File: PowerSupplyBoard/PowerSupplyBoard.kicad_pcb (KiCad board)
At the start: 4 copper layers, 50 x 80 mm, 70 parts, among them J101 BATTERY, J102 POWER, J103 USB_C, J104 PWR, J105 DATA, Q101 BSH205G2A, Q102 TD6790, Q103 TD6790, Q104 TD6790, U101 TPS63021, U102 MCP73834T, U103 TC7662Bx0A, U104 TC7662Bx0A, U105 CS5173

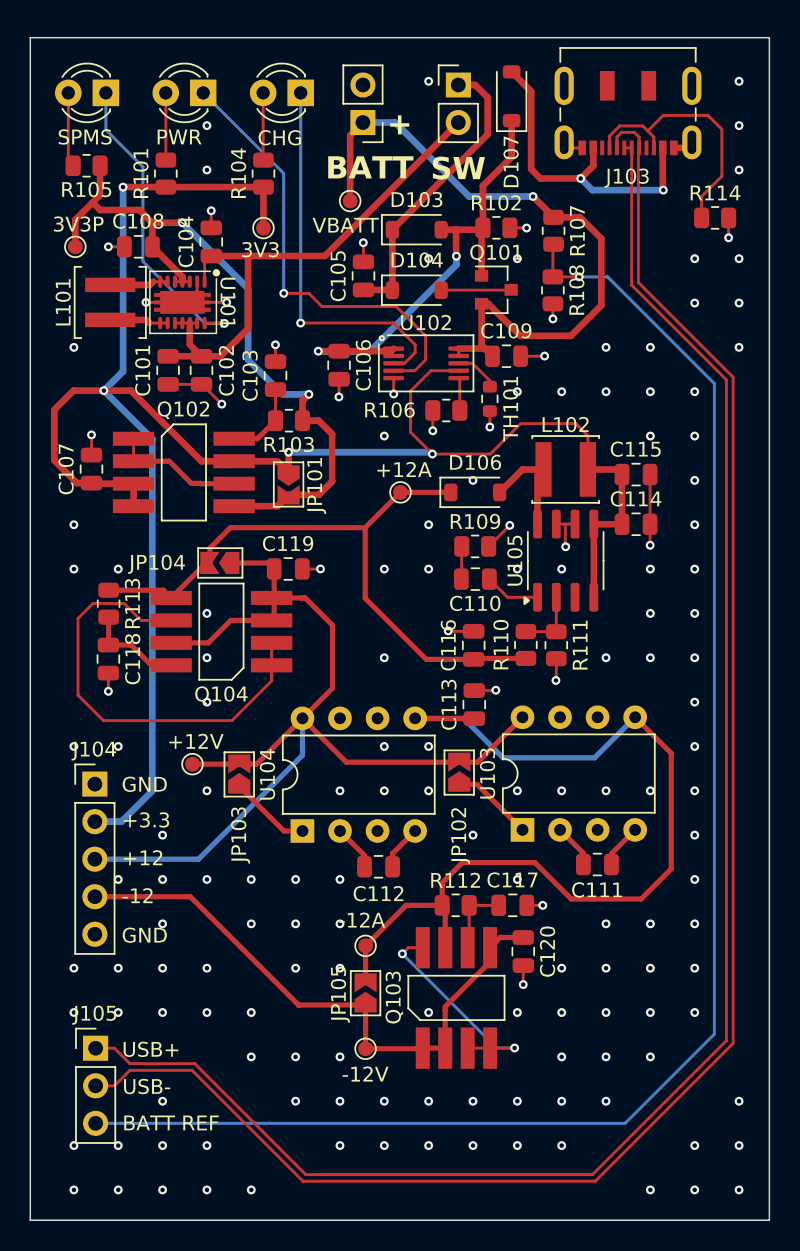
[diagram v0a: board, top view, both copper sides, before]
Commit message: Power Supply rev2
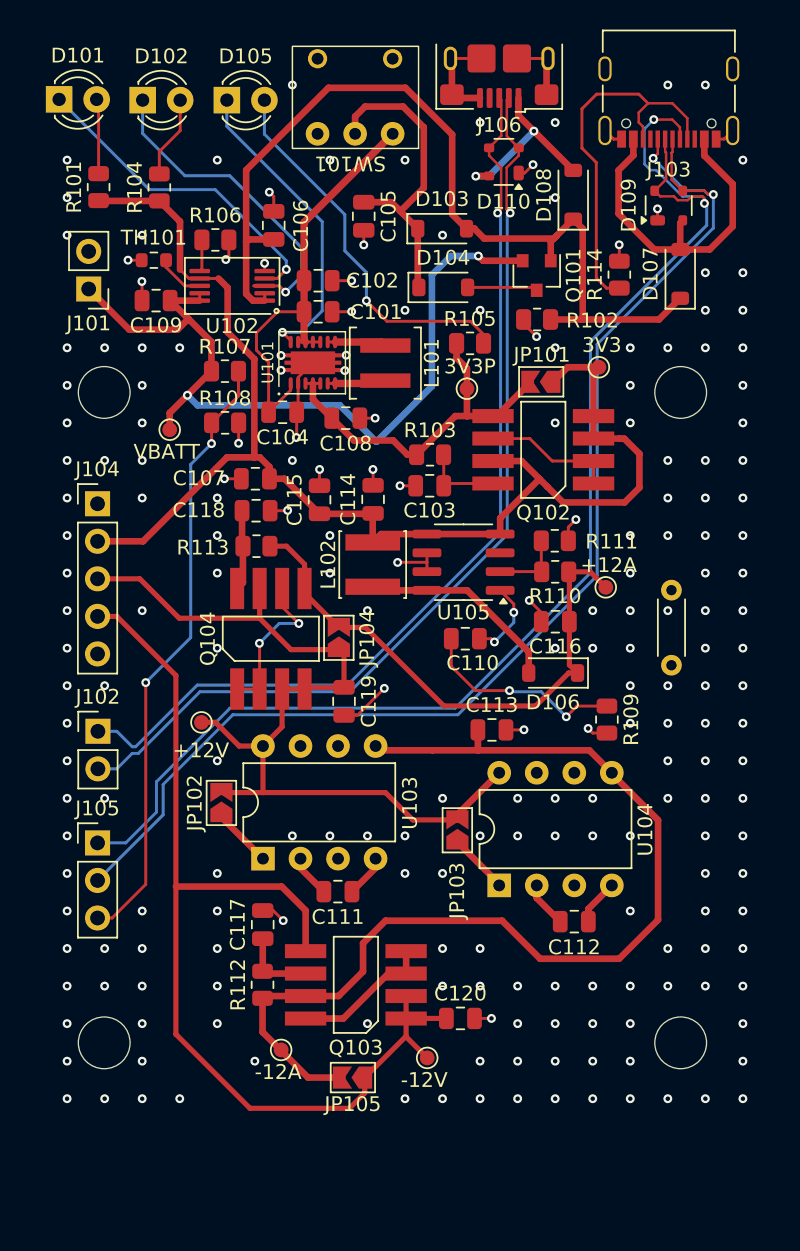
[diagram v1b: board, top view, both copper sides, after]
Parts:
- added D108: PMEG3030, Diode_SMD:D_SOD-123, F.Cu at (36.7, 10.6)
- added D109: SP0503BAHT, Package_TO_SOT_SMD:SOT-143, F.Cu at (43.2, 11.4)
- added D110: SP0503BAHT, Package_TO_SOT_SMD:SOT-143, F.Cu at (32.0, 8.40)
- added J106: USB_B_Micro, Connector_USB:USB_Micro-B_Amphenol_10118193-0001LF_Horizontal, F.Cu at (31.7, 1.41)
- added R115: LOOP, Resistor_THT:R_Axial_DIN0204_L3.6mm_D1.6mm_P5.08mm_Horizontal, F.Cu at (43.4, 42.5)
- added REF**: MountingHole_3.5mm, MountingHole:MountingHole_3.5mm, F.Cu at (44.0, 24.0)
- added REF**: MountingHole_3.5mm, MountingHole:MountingHole_3.5mm, F.Cu at (44.0, 68.0)
- added REF**: MountingHole_3.5mm, MountingHole:MountingHole_3.5mm, F.Cu at (5.00, 68.0)
- added REF**: MountingHole_3.5mm, MountingHole:MountingHole_3.5mm, F.Cu at (5.00, 24.0)
- added SW101: SW_SPDT, Button_Switch_THT:SW_NKK_B12JH_SPDT, F.Cu at (24.5, 6.50)
- J102: value POWER -> DATA2
- J103: footprint Connector_USB:USB_C_Receptacle_JAE_DX07S016JA1R1500 -> Connector_USB:USB_C_Receptacle_Palconn_UTC16-G
- J105: value DATA -> DATA1
- moved J102 50.1 mm to (4.58, 46.9)
- moved R105 28.6 mm to (29.8, 20.7), turned to 0 degrees
- moved TP102 28.2 mm to (29.5, 23.7)
- moved TH101 24.6 mm to (8.36, 15.1), turned to 180 degrees
- moved TP101 24.6 mm to (38.5, 22.3), turned to 0 degrees
- moved Q102 24.2 mm to (34.6, 27.9), turned to 180 degrees
- moved R107 24.2 mm to (13.2, 22.6), turned to 0 degrees
- moved C109 24.0 mm to (8.51, 17.8), turned to 180 degrees
- moved R108 23.9 mm to (13.2, 26.1), turned to 0 degrees
- moved J101 21.7 mm to (3.95, 17.0)
- moved C115 21.5 mm to (19.6, 31.3), turned to 90 degrees
- moved TP103 19.7 mm to (9.43, 26.5)
- moved R106 19.4 mm to (12.5, 13.7), turned to 0 degrees
- moved L101 19.1 mm to (24.0, 22.0), turned to -90 degrees
- moved J104 19.0 mm to (4.55, 31.5)
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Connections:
- J102 pad 1: VCC -> USBM_D+
- J102 pad 2: V_PWR -> USBM_D-
- J103 pad A6: USB_D+ -> USBC_D+
- J103 pad A7: USB_D- -> USBC_D-
- J103 pad B6: USB_D+ -> USBC_D+
- J103 pad B7: USB_D- -> USBC_D-
- J105 pad 1: USB_D+ -> USBC_D-
- J105 pad 2: USB_D- -> USBC_D+
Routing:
- net USB_D-: track 117.0 -> 0.00 mm
- net USB_D+: track 113.5 -> 0.00 mm
- net USBC_D-: track 0.00 -> 89.8 mm, vias 0 -> 2
- net USBC_D+: track 0.00 -> 85.1 mm, vias 0 -> 2
- net USBM_D-: track 0.00 -> 64.7 mm, vias 0 -> 1
- net USBM_D+: track 0.00 -> 64.0 mm, vias 0 -> 1
- net BATT_REF: track 104.5 -> 41.5 mm, vias 1 -> 2
- net +3.3V: track 135.9 -> 89.8 mm, vias 4 -> 0
- net -12V: track 40.3 -> 71.2 mm
- net VDD: track 33.6 -> 62.9 mm, vias 2 -> 0
- net +3.3VP: track 49.7 -> 25.6 mm, vias 2 -> 0
- net Net-(D105-A): track 5.06 -> 25.9 mm, vias 0 -> 1
- net Net-(Q104B-B2): track 29.9 -> 10.7 mm, vias 0 -> 2
- net GND: track 46.4 -> 59.6 mm, vias 162 -> 215
- net Net-(D108-A): track 0.00 -> 12.5 mm, vias 0 -> 2
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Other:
- board outline removed
- board text removed: "+"
- board text removed: "+12"
- board text removed: "+3.3"
- board text removed: "-12"
- board text removed: "BATT"
- board text removed: "BATT REF"
- board text removed: "CHG"
- board text removed: "GND"
- board text removed: "PWR"
- board text removed: "SPMS"
- board text removed: "SW"
- board text removed: "USB+"
- board text removed: "USB-"

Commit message: Power supply rev2 gerbers
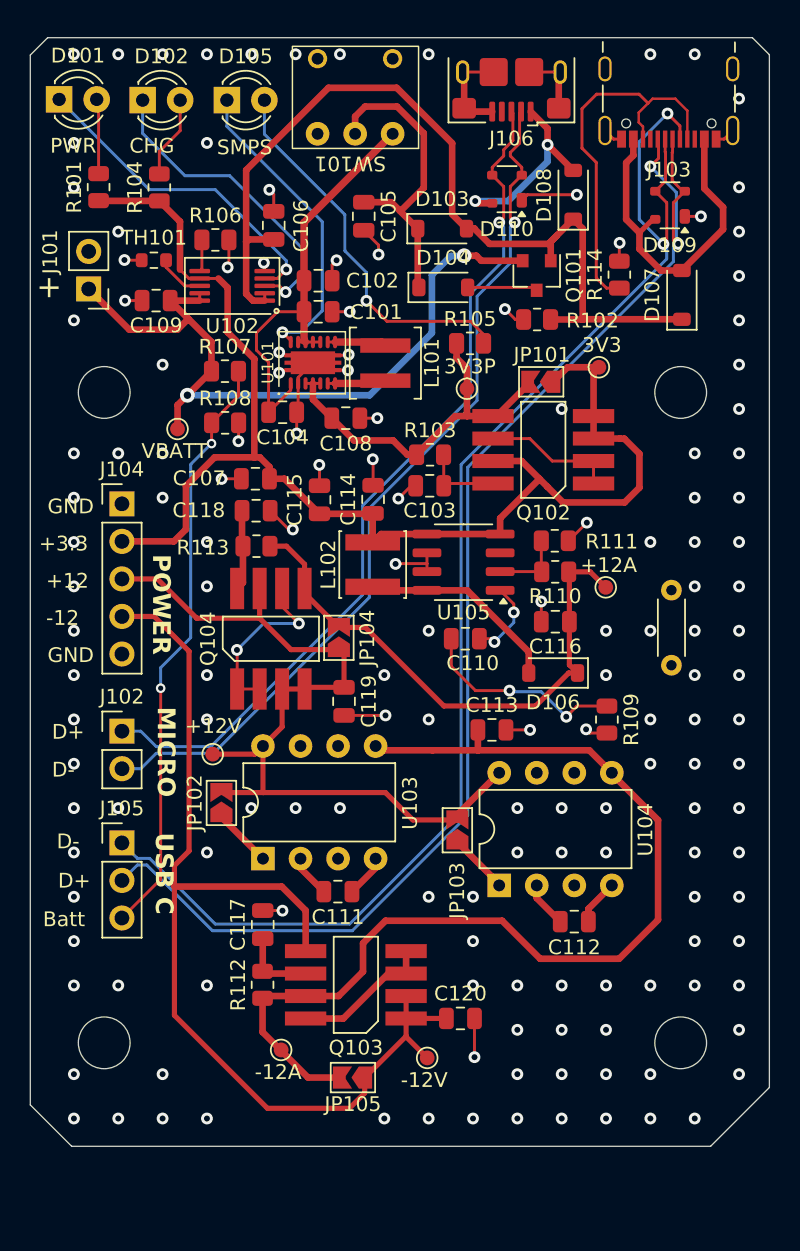
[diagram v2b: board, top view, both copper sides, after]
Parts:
- moved TP107 2.28 mm to (12.3, 48.5), turned to 0 degrees
- moved D110 1.86 mm to (32.2, 10.2)
- moved J104 1.65 mm to (6.20, 31.5)
- moved J105 1.65 mm to (6.20, 54.5)
- moved J102 1.63 mm to (6.20, 46.9)
- moved D107 1.42 mm to (44.1, 17.4)
- moved J106 1.24 mm to (32.5, 2.33)
- moved TP103 0.53 mm to (9.96, 26.5)
- moved D109 0.09 mm to (43.3, 11.3), turned to 180 degrees
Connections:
- D109 pad 2: Net-(D107-A) -> USBC_D+
- D109 pad 3: USBC_D+ -> USBC_D-
- D109 pad 4: USBC_D- -> Net-(D107-A)
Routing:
- net GND: track 59.6 -> 68.5 mm, vias 215 -> 155
- net USBM_D+: track 64.0 -> 58.8 mm
- net USBM_D-: track 64.7 -> 59.5 mm
- net VBATT: track 55.5 -> 50.5 mm
- net USBC_D+: track 85.1 -> 89.5 mm
- net USBC_D-: track 89.8 -> 92.9 mm
- net +12V: track 60.7 -> 57.9 mm
- net Net-(D102-K): track 22.7 -> 21.3 mm
- net BATT_REF: track 41.5 -> 40.3 mm
- net Net-(Q104B-B2): track 10.7 -> 11.9 mm
- net Net-(D108-A): track 12.5 -> 13.5 mm
- net Net-(J103-CC1): track 26.1 -> 26.7 mm
- net VDD: track 62.9 -> 62.4 mm
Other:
- board outline added: 50 x 75 mm
- board text added: "+"
- board text added: "+12"
- board text added: "+3.3"
- board text added: "-12"
- board text added: "Batt"
- board text added: "CHG"
- board text added: "D+"
- board text added: "D-"
- board text added: "GND"
- board text added: "MICRO"
- board text added: "POWER"
- board text added: "PWR"
- board text added: "Rev. 2 July 2024 Hayden Setlik"
- board text added: "SMPS"
- board text added: "USB C"
- board text added: "USB Synth Power Supply"
